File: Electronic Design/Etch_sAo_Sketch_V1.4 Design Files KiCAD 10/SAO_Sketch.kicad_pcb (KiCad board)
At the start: 2 copper layers, 38.1 x 50.8 mm, 14 parts, among them U1 LIS3DHTR, X1 SAO_conn_SFH11-NBPC-D03-ST-BK, X2 OLED_128x128

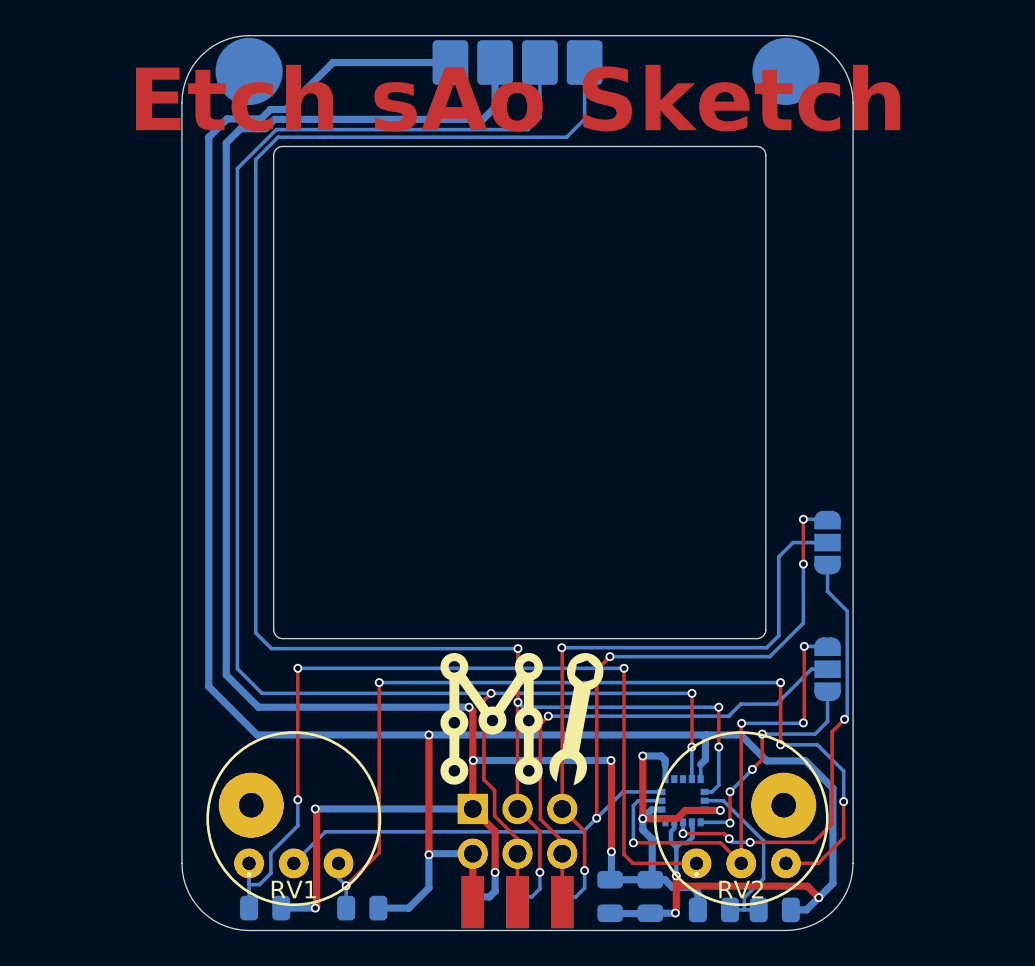
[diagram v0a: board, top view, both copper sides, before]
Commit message: Add V1.4.0 hardware design
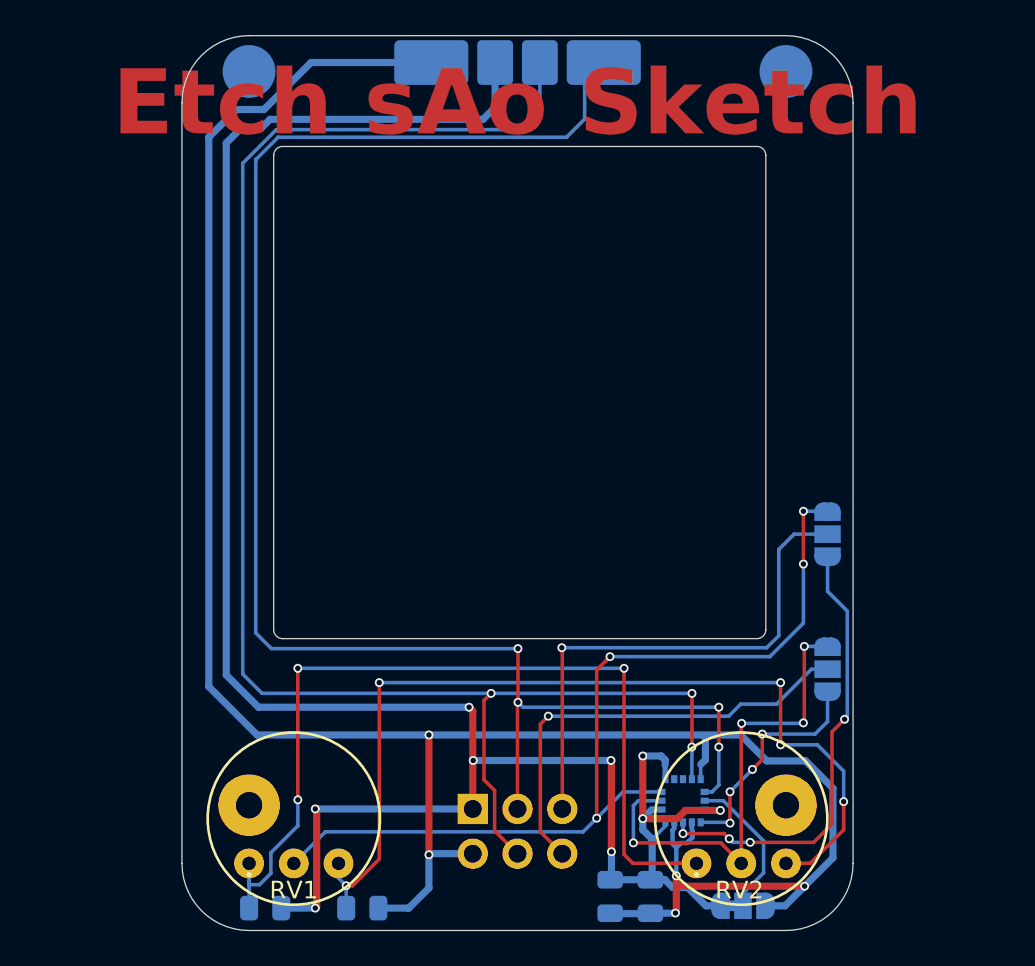
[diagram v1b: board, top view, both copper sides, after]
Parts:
- removed L3: Core_64_Logo, Andy_Footprint_Library:Machine_Ideas_logo
- removed R3, R4: 10K, Resistor_SMD:R_0805_2012Metric
- added JP5: SolderJumper_3_Bridged12, Jumper:SolderJumper-3_P1.3mm_Bridged12_RoundedPad1.0x1.5mm_NumberLabels, B.Cu at (93.6, 148.6)
- X1: value SAO_conn_SFH11-NBPC-D03-ST-BK -> SAO MALE HEADER; footprint Andy_Footprint_Library:Badgelife-SAOv169-BADGE-2x3-Edge-Connect-no-front-text-shortened -> Andy_Footprint_Library:Badgelife-SAOv169-BADGE-2x3-PINS-SHROUD-no-front-text
- moved JP3 0.48 mm to (98.5, 127.5)
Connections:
- C1 pad 1: VIN -> /3V3
- C2 pad 1: VIN -> /3V3
- R5 pad 1: VIN -> /3V3
- U1 pad 1: VIN -> /3V3
- U1 pad 13: unconnected-(U1-ADC3-Pad13) -> /3V3
- U1 pad 14: VIN -> /3V3
- U1 pad 8: VIN -> /3V3
- X1 pad 1: VIN -> /3V3
- X2 pad 2: VIN -> /3V3
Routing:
- net VIN: track 129.8 -> 0.00 mm, vias 10 -> 0
- net /3V3: track 0.00 -> 125.0 mm, vias 0 -> 9
- net /SDA: track 97.5 -> 91.0 mm, vias 5 -> 4
- net /GPIO1: track 35.8 -> 29.8 mm, vias 2 -> 1
- net GND: track 132.0 -> 128.8 mm
- net /SCL: track 93.7 -> 91.0 mm
- net /GPIO2: track 27.9 -> 25.5 mm
- net Net-(JP5-C): track 10.3 -> 8.46 mm
- net /POT1L: track 51.4 -> 52.3 mm
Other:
- board text added: "A=0x19 O=0x3C"
- board text added: "^"
- board text removed: "ACL 0x19 OLED 0x3C"
